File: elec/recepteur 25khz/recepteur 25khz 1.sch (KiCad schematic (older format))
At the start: 15 parts, among them P1 CONN_6, P10 CONN_6, P11 CONN_7, P14 CONN_7, P15 CONN_7, P16 CONN_7, P17 CONN_6, P18 CONN_7, P19 CONN_5, P20 CONN_7, P21 CONN_7, P4 CONN_6, P5 CONN_6, P8 CONN_6, P9 CONN_5

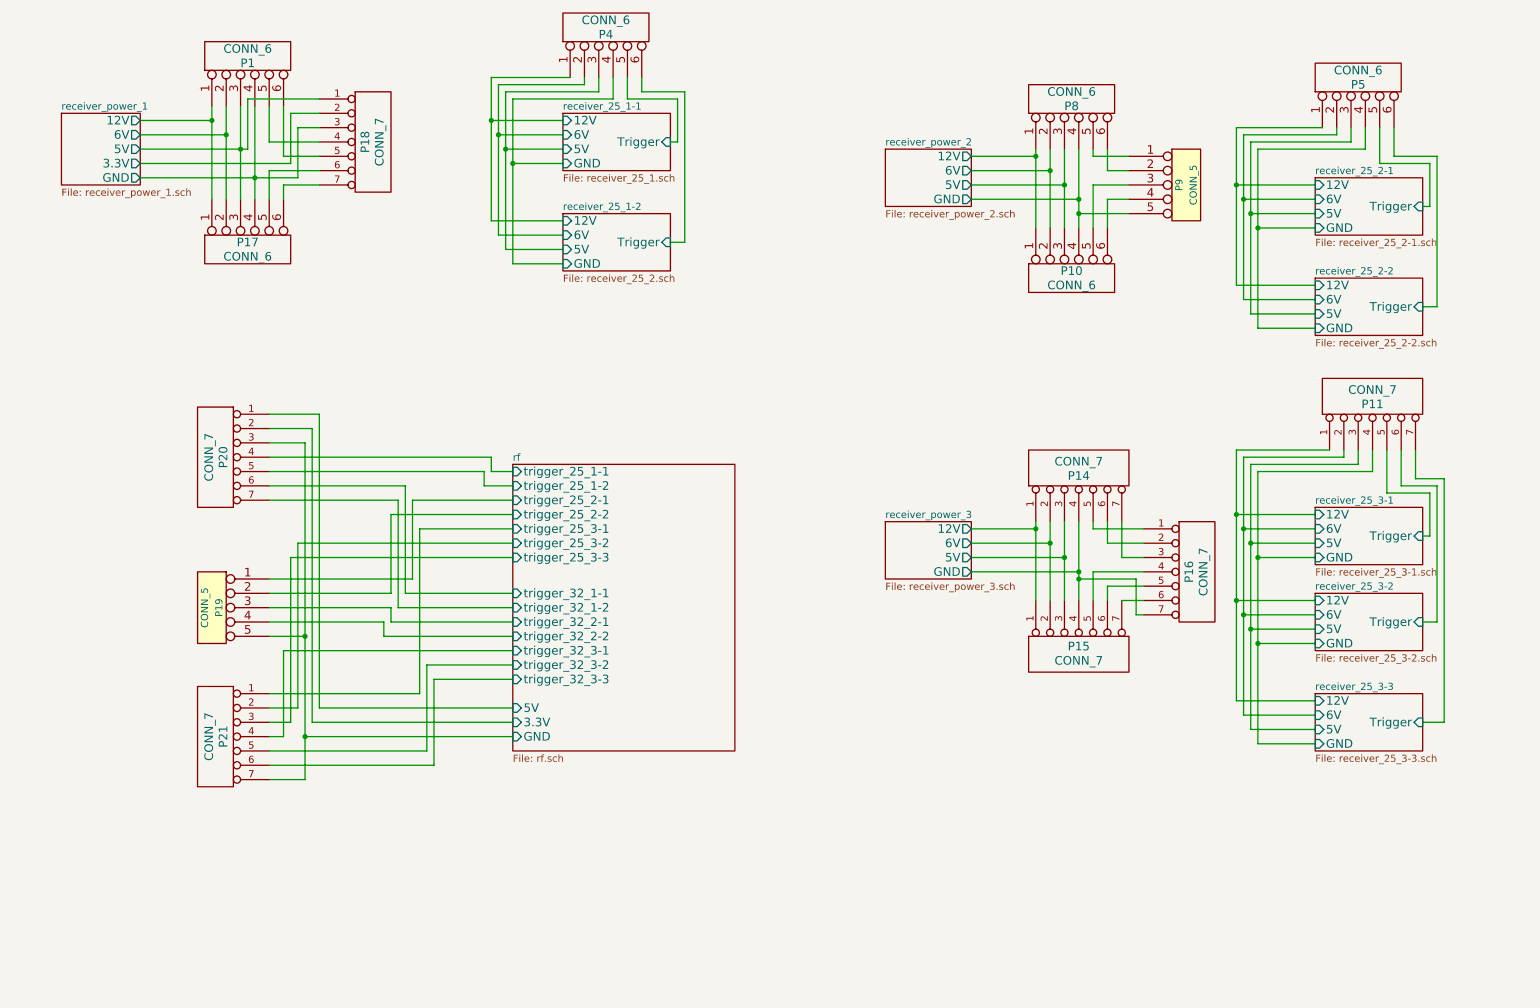
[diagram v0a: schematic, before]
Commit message: Add some documentation
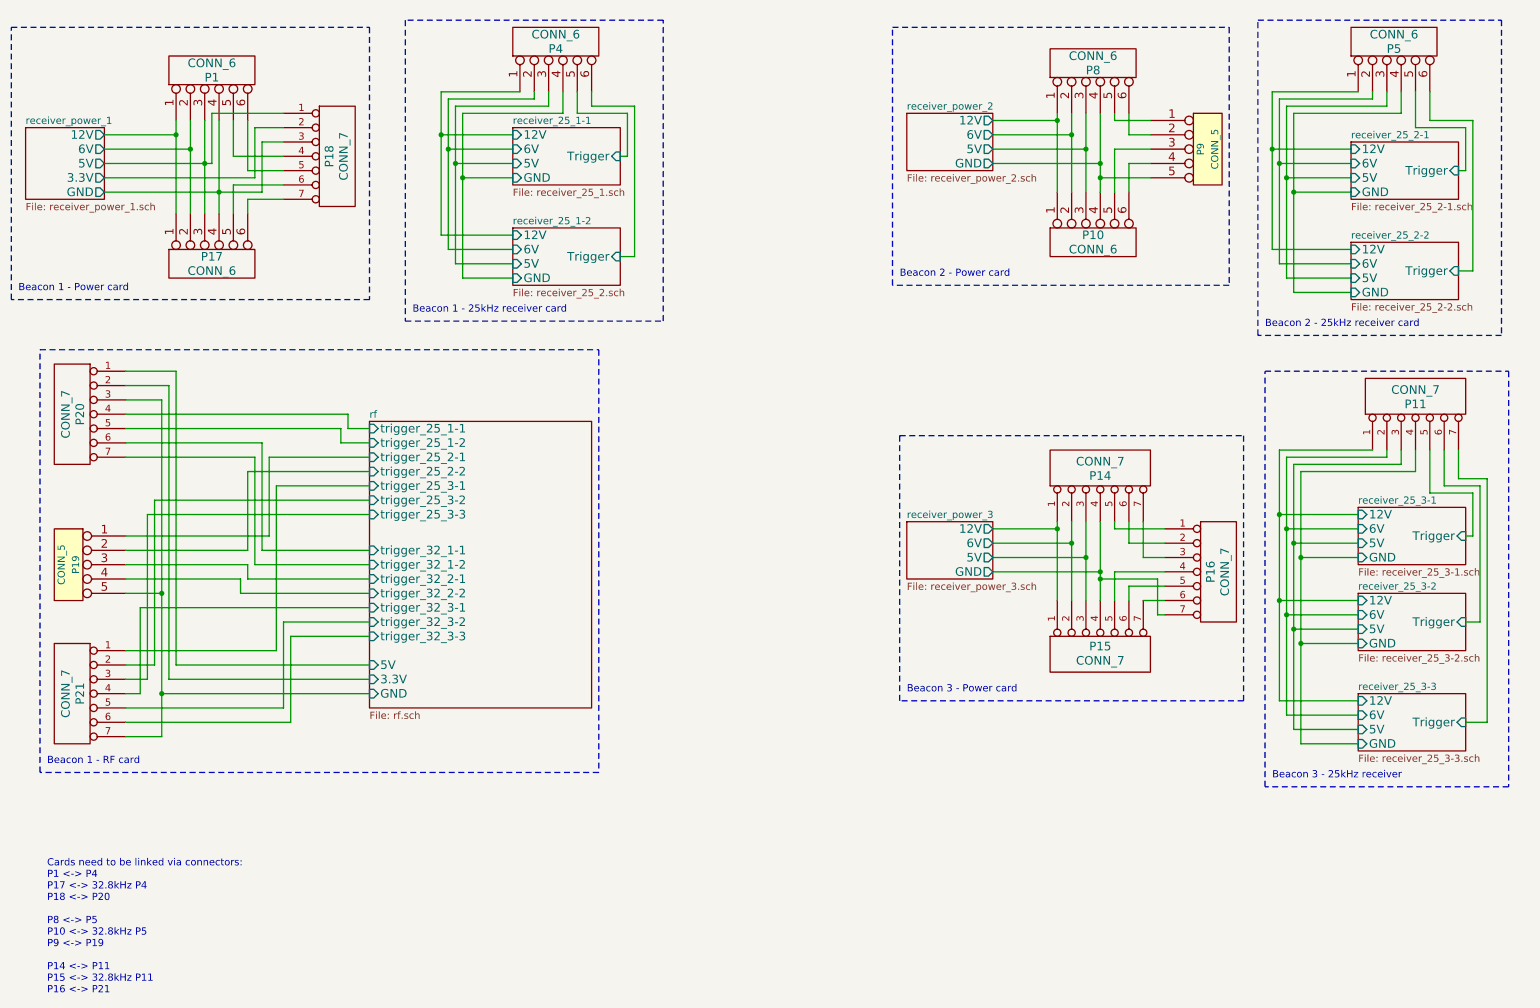
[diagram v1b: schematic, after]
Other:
- note added: "Beacon 1 - 25kHz receiver card"
- note added: "Beacon 1 - Power card"
- note added: "Beacon 1 - RF card"
- note added: "Beacon 2 - 25kHz receiver card"
- note added: "Beacon 2 - Power card"
- note added: "Beacon 3 - 25kHz receiver"
- note added: "Beacon 3 - Power card"
- note added: "Cards need to be linked via connectors:\nP1 <-> P4\nP17 <-> 32.8kHz P4\nP18 <-> P20\n\nP8 <-> P5\nP10 <-> 32.8kHz P5\nP9 <-> P19\n\nP14 <-> P11\nP15 <-> 32.8kHz P11\nP16 <-> P21"
- moved on the sheet: P1, P10, P11, P14, P15, P16, P17, P18, P19, P20, P21, P4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
